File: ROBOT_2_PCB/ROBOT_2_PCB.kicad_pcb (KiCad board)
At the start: 2 copper layers, 31 parts, among them J1 Bluetooth, U1 ULN2003

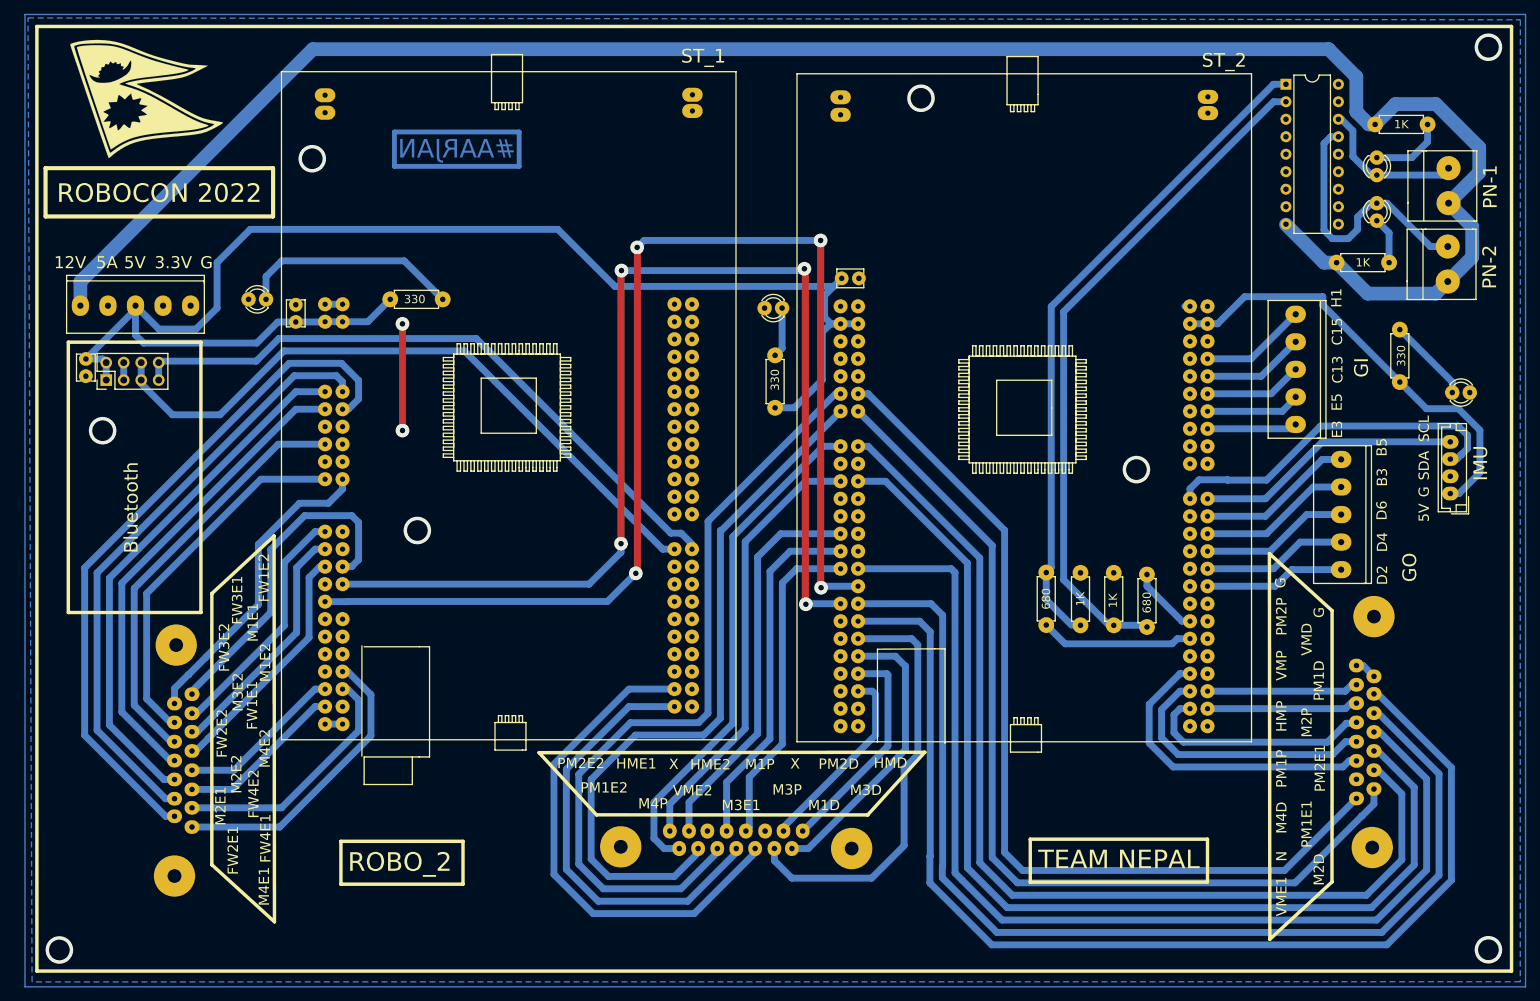
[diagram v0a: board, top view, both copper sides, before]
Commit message: Finally Created1
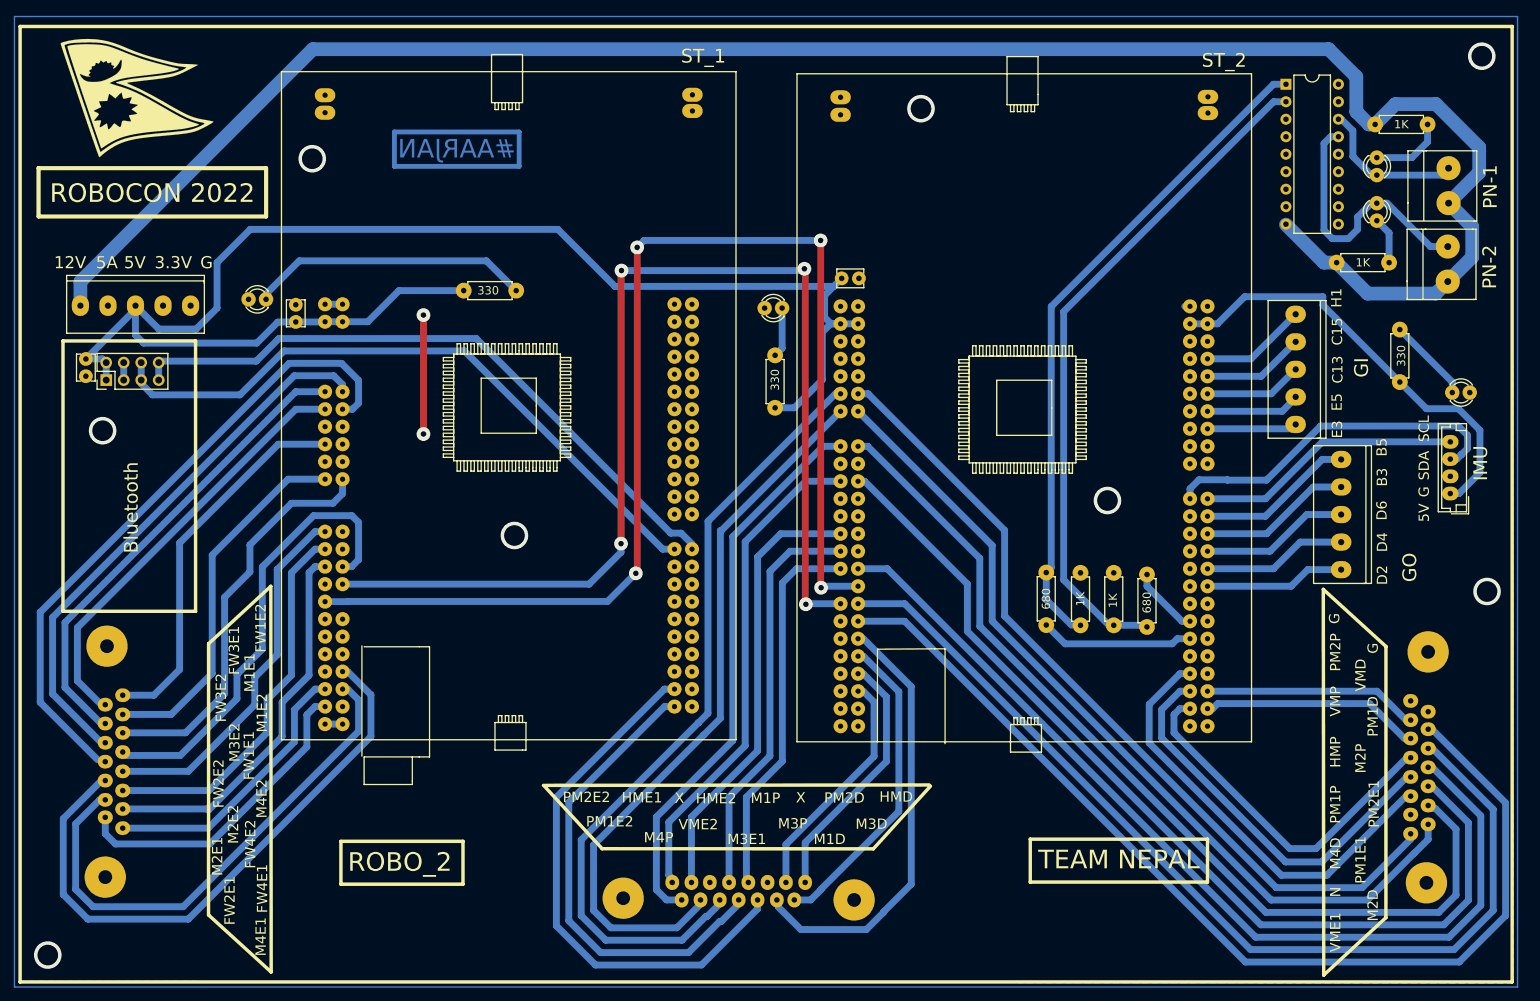
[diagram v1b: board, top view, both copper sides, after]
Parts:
- moved S1I1 10.7 mm to (96.0, 60.2)
- moved db-1 10.1 mm to (46.5, 138.2)
- moved db-3 9.39 mm to (233.5, 119.8)
- moved db-2 7.47 mm to (145.6, 146.1)
- moved NEPAL1 1.40 mm to (47.5, 34.5)
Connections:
- db-1 pad 1: Motor_4_Enc_1 -> Motor_4_Enc_2
- db-1 pad 10: Motor_2_Enc_1 -> FW4_E1
- db-1 pad 11: Motor_2_Enc_2 -> Motor_4_Enc_1
- db-1 pad 12: FW2_E2 -> FW2_E1
- db-1 pad 13: Motor_3_Enc_2 -> Motor_2_Enc_1
- db-1 pad 14: FW3_E2 -> Motor_2_Enc_2
- db-1 pad 15: FW3_E1 -> FW2_E2
- db-1 pad 2: FW4_E1 -> FW1_E1
- db-1 pad 3: FW4_E2 -> Motor_1_Enc_2
- db-1 pad 4: Motor_4_Enc_2 -> Motor_1_Enc_1
- db-1 pad 5: FW1_E1 -> FW1_E2
- db-1 pad 6: Motor_1_Enc_2 -> FW3_E1
- db-1 pad 7: Motor_1_Enc_1 -> FW3_E2
- db-1 pad 8: FW1_E2 -> Motor_3_Enc_2
- db-1 pad 9: FW2_E1 -> FW4_E2
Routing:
- net Motor_4_Enc_1: track 43.0 -> 88.1 mm
- net FW4_E1: track 36.3 -> 75.5 mm
- net FW4_E2: track 24.3 -> 45.9 mm
- net FW1_E1: track 35.5 -> 55.8 mm
- net Motor_1_Enc_2: track 35.8 -> 55.4 mm
- net Picker_Motor1_PWM: track 39.4 -> 58.1 mm
- net Horizontal_Motor_PWM: track 33.6 -> 52.1 mm
- net Motor_4_DIR: track 45.8 -> 64.1 mm
- net Motor_2_Pwm: track 155.9 -> 138.1 mm
- net Motor_1_Enc_1: track 35.6 -> 53.4 mm
- net FW1_E2: track 49.1 -> 66.8 mm
- net Motor_4_Enc_2: track 24.9 -> 41.2 mm
- net Picker_Motor1_DIR: track 157.8 -> 143.2 mm
- net Picker_Motor2_E1: track 154.2 -> 140.1 mm
- net FW3_E1: track 45.2 -> 58.9 mm
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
